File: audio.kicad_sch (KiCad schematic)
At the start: 6 parts, among them J6 AudioJack3, U8 LM386

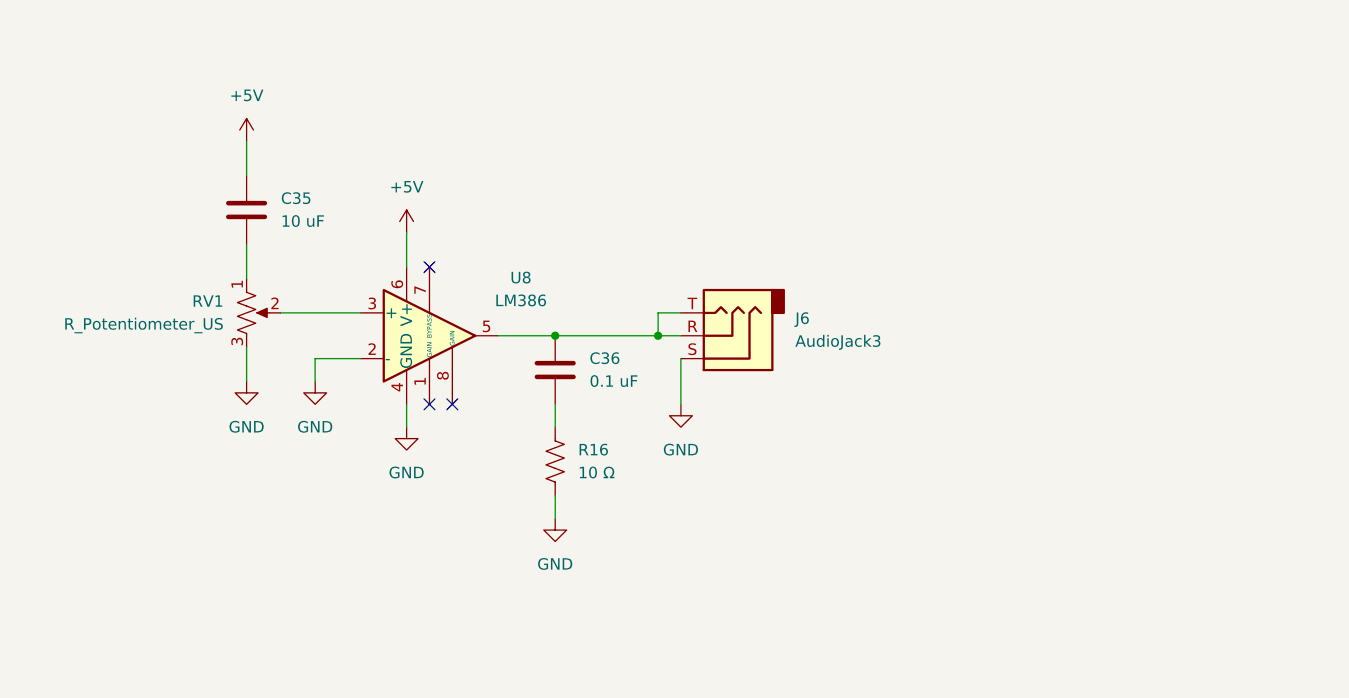
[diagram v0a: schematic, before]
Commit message: Updated Schematic
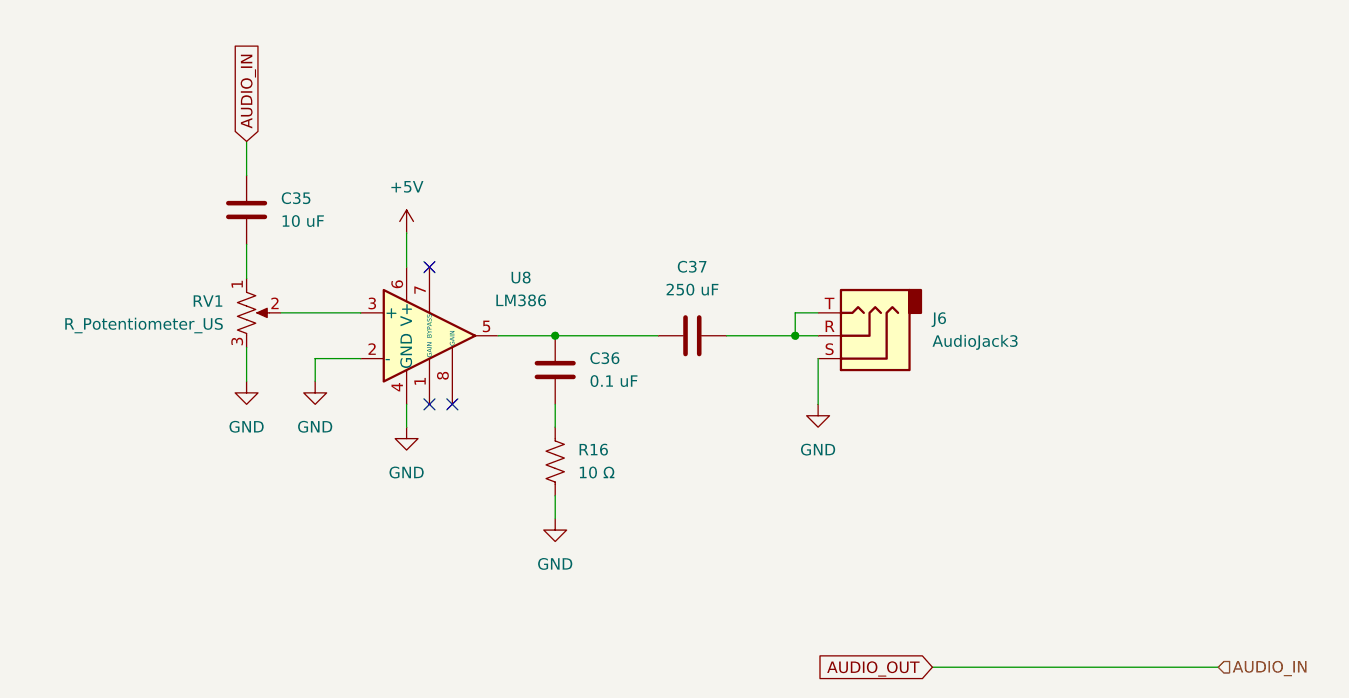
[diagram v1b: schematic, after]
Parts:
- added C37: 250 uF, Capacitor_SMD:C_0805_2012Metric, symbol Device:C
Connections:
- net +5V: no longer C35.2
- net at C36.2, U8.5: now also C37.1; no longer J6.R, J6.T
- new net: C37.2, J6.R, J6.T
- new net AUDIO_IN: C35.2
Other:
- moved on the sheet: J6
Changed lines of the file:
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@@
 	(paper "A4")
 	(junction
-		(at 168.91 86.36)
+		(at 184.15 86.36)
 		(diameter 0)
 		(color 0 0 0 0)
@@
 	(wire
 		(pts
-			(xy 168.91 83.82) (xy 168.91 86.36)
+			(xy 184.15 83.82) (xy 184.15 86.36)
 		)
 		(stroke
@@
 	(wire
 		(pts
+			(xy 176.53 86.36) (xy 184.15 86.36)
+		)
+		(stroke
+			(width 0)
+			(type default)
+		)
+	)
+	(wire
+		(pts
 			(xy 135.89 88.9) (xy 130.81 88.9)
 		)
@@
 	(wire
 		(pts
-			(xy 171.45 88.9) (xy 171.45 93.98)
-		)
-		(stroke
-			(width 0)
-			(type default)
-		)
-	)
-	(wire
-		(pts
-			(xy 171.45 83.82) (xy 168.91 83.82)
+			(xy 186.69 88.9) (xy 186.69 93.98)
+		)
+		(stroke
+			(width 0)
+			(type default)
+		)
+	)
+	(wire
+		(pts
+			(xy 186.69 83.82) (xy 184.15 83.82)
+		)
+		(stroke
+			(width 0)
+			(type default)
+		)
+	)
+	(wire
+		(pts
+			(xy 199.39 123.19) (xy 231.14 123.19)
 		)
 		(stroke
@@
 	(wire
 		(pts
-			(xy 168.91 86.36) (xy 171.45 86.36)
+			(xy 184.15 86.36) (xy 186.69 86.36)
 		)
 		(stroke
@@
 		)
 	)
-	(symbol
-		(lib_id "power:+5V")
-		(at 123.19 64.77 0)
-		(unit 1)
-		(exclude_from_sim no)
-		(in_bom yes)
-		(on_board yes)
-		(dnp no)
-		(fields_autoplaced yes)
-		(property "Reference" "#PWR072"
-			(at 123.19 68.58 0)
-			(effects
-				(font
-					(size 1.27 1.27)
-				)
-				(hide yes)
-			)
-		)
-		(property "Value" "+5V"
-			(at 123.19 59.69 0)
-			(effects
-				(font
-					(size 1.27 1.27)
-				)
-			)
-		)
-		(property "Footprint" ""
-			(at 123.19 64.77 0)
-			(effects
-				(font
-					(size 1.27 1.27)
-				)
-				(hide yes)
-			)
-		)
-		(property "Datasheet" ""
-			(at 123.19 64.77 0)
-			(effects
-				(font
-					(size 1.27 1.27)
-				)
-				(hide yes)
-			)
-		)
-		(property "Description" "Power symbol creates a global label with name \"+5V\""
-			(at 123.19 64.77 0)
-			(effects
-				(font
-					(size 1.27 1.27)
-				)
-				(hide yes)
-			)
-		)
-		(pin "1"
-		)
-		(instances
-			(project ""
-				(path "/35c074f0-8545-4dc1-a57d-3ef0bc7d9188/b0fb54ab-b2e8-4f49-90f2-51362383cff9"
-					(reference "#PWR072")
-					(unit 1)
-				)
-			)
+	(global_label "AUDIO_OUT"
+		(shape input)
+		(at 199.39 123.19 180)
+		(fields_autoplaced yes)
+		(effects
+			(font
+				(size 1.27 1.27)
+			)
+			(justify right)
+		)
+		(property "Intersheetrefs" "${INTERSHEET_REFS}"
+			(at 186.1842 123.19 0)
+			(effects
+				(font
+					(size 1.27 1.27)
+				)
+				(justify right)
+				(hide yes)
+			)
+		)
+	)
+	(global_label "AUDIO_IN"
+		(shape input)
+		(at 123.19 64.77 90)
+		(fields_autoplaced yes)
+		(effects
+			(font
+				(size 1.27 1.27)
+			)
+			(justify left)
+		)
+		(property "Intersheetrefs" "${INTERSHEET_REFS}"
+			(at 123.19 53.2575 90)
+			(effects
+				(font
+					(size 1.27 1.27)
+				)
+				(justify left)
+				(hide yes)
+			)
+		)
+	)
+	(hierarchical_label "AUDIO_IN"
+		(shape input)
+		(at 231.14 123.19 0)
+		(effects
+			(font
+				(size 1.27 1.27)
+			)
+			(justify left)
 		)
 	)
@@
 	(symbol
 		(lib_id "power:GND")
-		(at 171.45 93.98 0)
+		(at 186.69 93.98 0)
 		(unit 1)
 		(exclude_from_sim no)
@@
 		(fields_autoplaced yes)
 		(property "Reference" "#PWR071"
-			(at 171.45 100.33 0)
+			(at 186.69 100.33 0)
 			(effects
 				(font
@@
 		)
 		(property "Value" "GND"
-			(at 171.45 99.06 0)
+			(at 186.69 99.06 0)
 			(effects
 				(font
@@
 		)
 		(property "Footprint" ""
-			(at 171.45 93.98 0)
+			(at 186.69 93.98 0)
 			(effects
 				(font
@@
 		)
 		(property "Datasheet" ""
-			(at 171.45 93.98 0)
+			(at 186.69 93.98 0)
 			(effects
 				(font
@@
 		)
 		(property "Description" "Power symbol creates a global label with name \"GND\" , ground"
-			(at 171.45 93.98 0)
+			(at 186.69 93.98 0)
 			(effects
 				(font
@@
 	(symbol
 		(lib_id "Connector_Audio:AudioJack3")
-		(at 176.53 86.36 180)
+		(at 191.77 86.36 180)
 		(unit 1)
 		(exclude_from_sim no)
@@
 		(fields_autoplaced yes)
 		(property "Reference" "J6"
-			(at 184.15 84.4549 0)
+			(at 199.39 84.4549 0)
 			(effects
 				(font
@@
 		)
 		(property "Value" "AudioJack3"
-			(at 184.15 86.9949 0)
+			(at 199.39 86.9949 0)
 			(effects
 				(font
@@
 		)
 		(property "Footprint" "Connector_Audio:Jack_3.5mm_CUI_SJ-3523-SMT_Horizontal"
-			(at 176.53 86.36 0)
+			(at 191.77 86.36 0)
 			(effects
 				(font
@@
 		)
 		(property "Datasheet" "~"
-			(at 176.53 86.36 0)
+			(at 191.77 86.36 0)
 			(effects
 				(font
@@
 		)
 		(property "Description" "Audio Jack, 3 Poles (Stereo / TRS)"
-			(at 176.53 86.36 0)
+			(at 191.77 86.36 0)
 			(effects
 				(font
@@
 					(unit 1)
 				)
+			)
+		)
+	)
+	(symbol
+		(lib_id "Device:C")
+		(at 172.72 86.36 90)
+		(unit 1)
+		(exclude_from_sim no)
+		(in_bom yes)
+		(on_board yes)
+		(dnp no)
+		(fields_autoplaced yes)
+		(property "Reference" "C37"
+			(at 172.72 78.74 90)
+			(effects
+				(font
+					(size 1.27 1.27)
+				)
+			)
+		)
+		(property "Value" "250 uF"
+			(at 172.72 81.28 90)
+			(effects
+				(font
+					(size 1.27 1.27)
+				)
+			)
+		)
+		(property "Footprint" "Capacitor_SMD:C_0805_2012Metric"
+			(at 176.53 85.3948 0)
+			(effects
+				(font
+					(size 1.27 1.27)
+				)
+				(hide yes)
+			)
+		)
+		(property "Datasheet" "~"
+			(at 172.72 86.36 0)
+			(effects
+				(font
+					(size 1.27 1.27)
+				)
+				(hide yes)
+			)
+		)
+		(property "Description" "Unpolarized capacitor"
+			(at 172.72 86.36 0)
+			(effects
+				(font
+					(size 1.27 1.27)
+				)
+				(hide yes)
+			)
+		)
+		(pin "1"
+		)
+		(pin "2"
+		)
+		(instances
+			(project ""
+				(path "/35c074f0-8545-4dc1-a57d-3ef0bc7d9188/b0fb54ab-b2e8-4f49-90f2-51362383cff9"
+					(reference "C37")
+					(unit 1)
+				)

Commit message: Updated Schematic
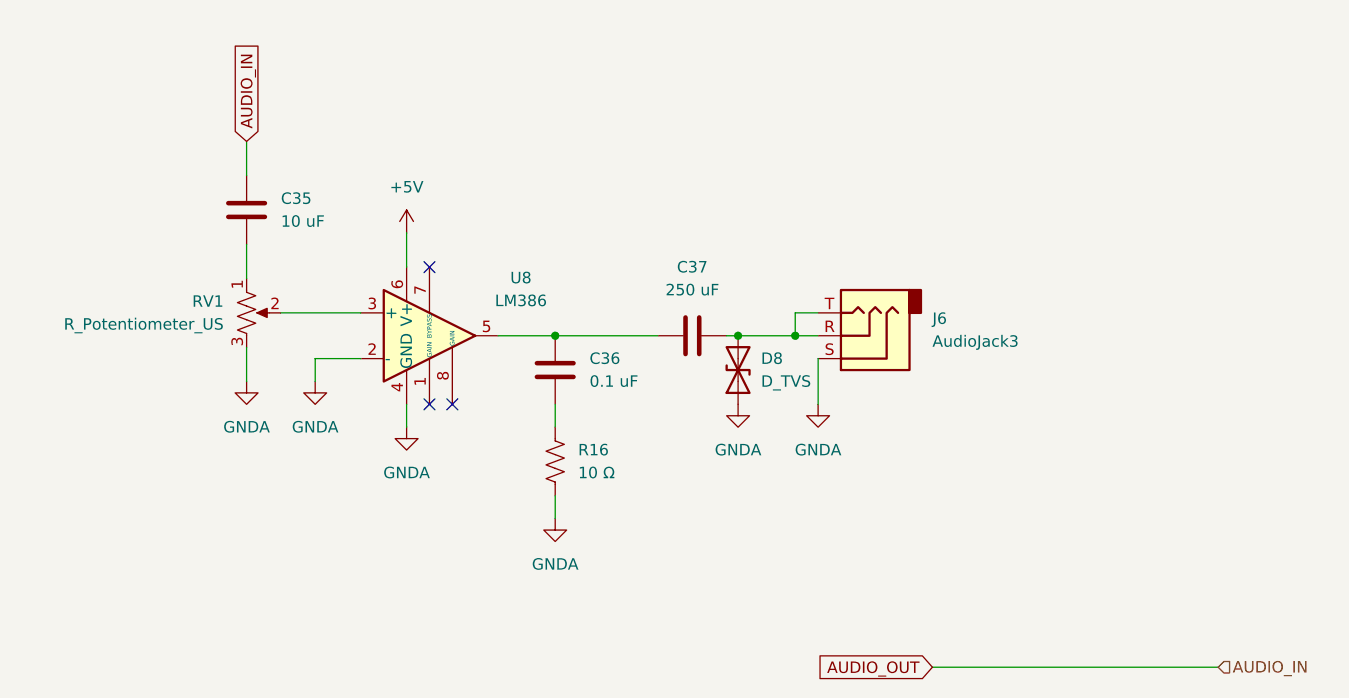
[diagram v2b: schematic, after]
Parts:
- added D8: D_TVS, symbol Device:D_TVS
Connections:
- net at C37.2, J6.R, J6.T: now also D8.2 (A2)
- net GND renamed GNDA
- net GNDA: now also D8.1 (A1)
